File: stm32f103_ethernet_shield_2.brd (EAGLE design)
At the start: 85.1 x 75.9 mm, 6 parts

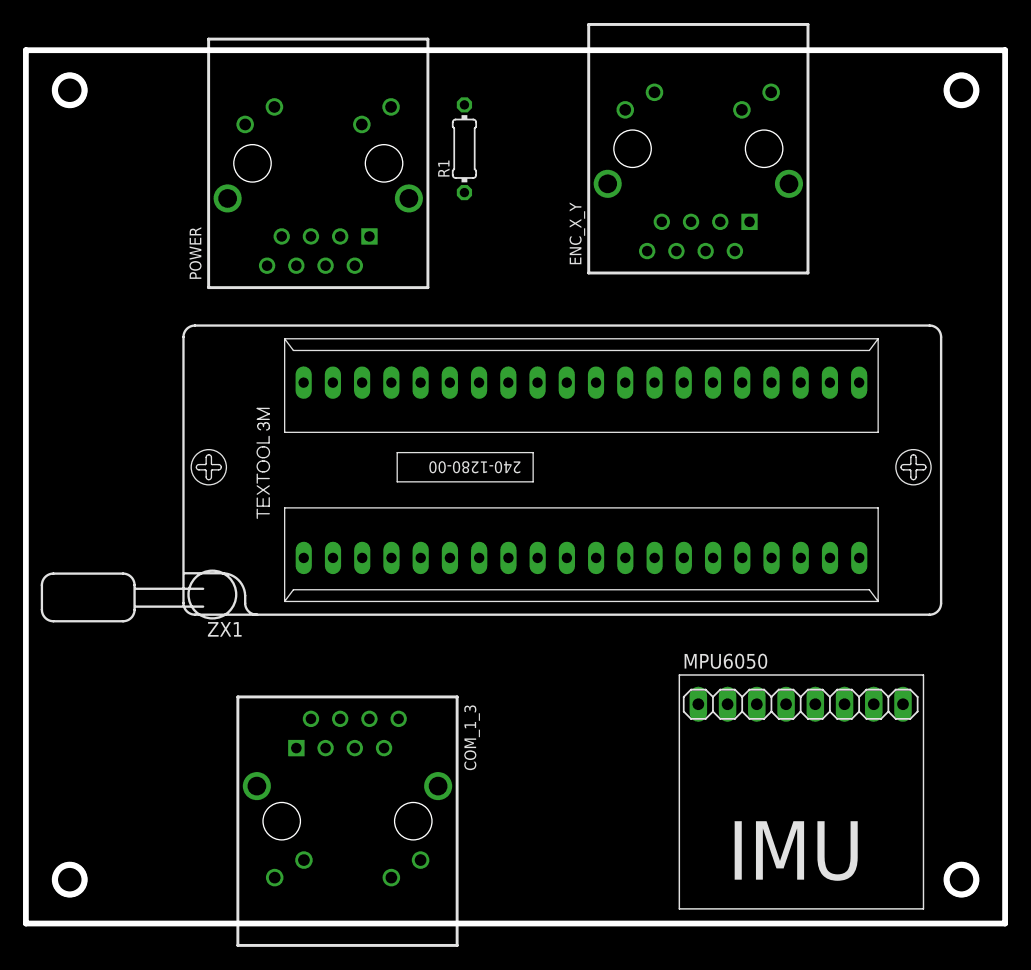
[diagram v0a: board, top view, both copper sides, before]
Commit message: Added a second design
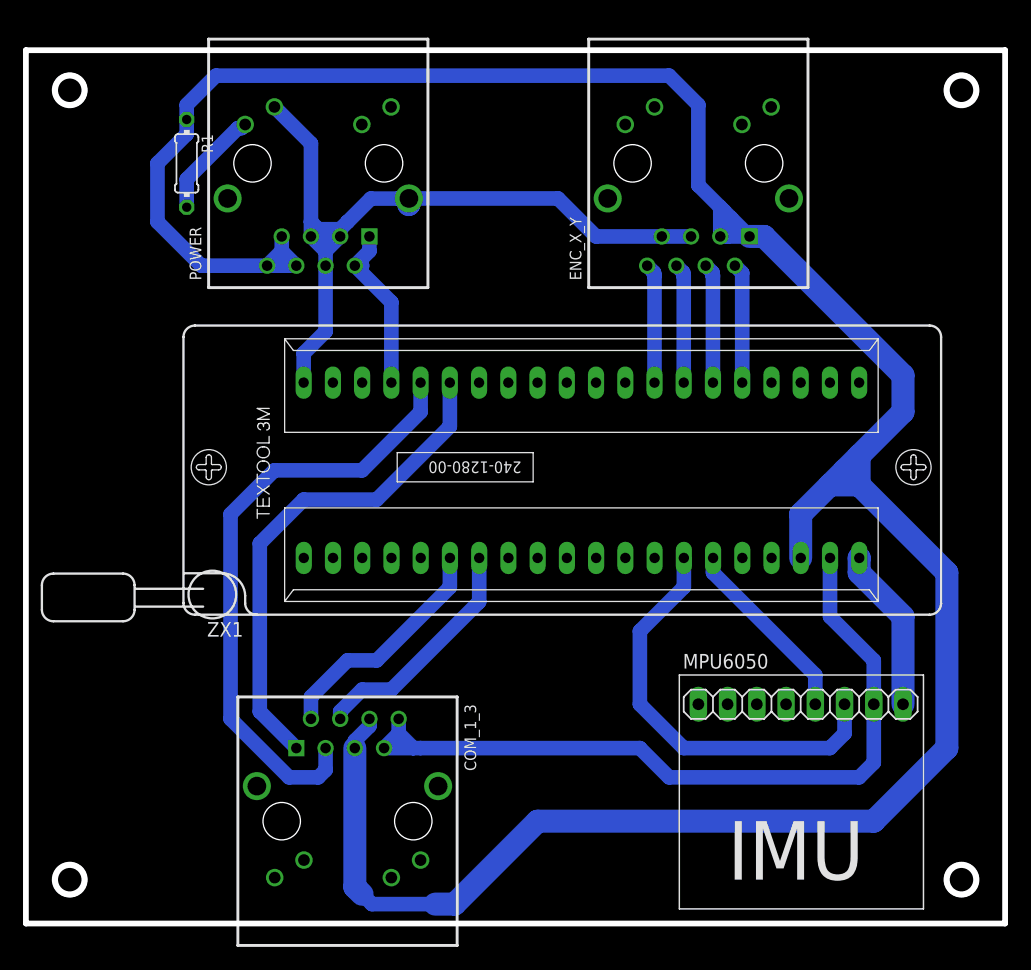
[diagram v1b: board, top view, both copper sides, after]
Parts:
- R1: value 150K -> 150R
- moved R1 24.2 mm to (14.0, 66.0), turned to 270 degrees
- moved ENC_X_Y 1.27 mm to (58.4, 66.0)
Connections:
- removed net LA1: POWER.9, R1.2
- new net RA1: POWER.12, R1.2
- net 5V: now also POWER.6, POWER.7, POWER.8; no longer POWER.1, POWER.2, POWER.3
- net GND@1: now also COM_1_3.7, COM_1_3.8; no longer POWER.10, POWER.4, POWER.5, POWER.6
- net GND@2: no longer ENC_X_Y.5, ENC_X_Y.7
- net GND@3: now also ENC_X_Y.5, ENC_X_Y.7, POWER.11, POWER.3, POWER.4, POWER.5, POWER.S2; no longer COM_1_3.7, COM_1_3.8
- net PA_10: now also COM_1_3.4; no longer COM_1_3.3
- net PA_9: now also COM_1_3.2; no longer COM_1_3.1
- net PB_10: now also COM_1_3.1; no longer COM_1_3.2
- net PB_11: now also COM_1_3.3; no longer COM_1_3.4
- net RESET: now also POWER.1, POWER.2; no longer POWER.7, POWER.8
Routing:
- net 5V: track 0.00 -> 240.4 mm
- net GND@1: track 0.00 -> 68.3 mm
- net GND@3: track 0.00 -> 67.9 mm
- net PB_11: track 0.00 -> 53.0 mm
- net PB_10: track 0.00 -> 43.6 mm
- net PB_6: track 0.00 -> 36.7 mm
- net PA_9: track 0.00 -> 20.5 mm
- net PA_10: track 0.00 -> 20.5 mm
- net PB_7: track 0.00 -> 16.4 mm
- net RESET: track 0.00 -> 15.8 mm
- net 3V3@1: track 0.00 -> 14.3 mm
- net PA_0: track 0.00 -> 10.4 mm
- net PA_3: track 0.00 -> 10.4 mm
- net PA_2: track 0.00 -> 10.4 mm
- net PA_1: track 0.00 -> 10.4 mm
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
